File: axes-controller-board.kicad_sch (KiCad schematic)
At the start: 58 parts, among them IC1 TPS5450QDDARQ1, J10 Conn_01x08, J11 Conn_01x04, J12 Conn_01x08, J13 Conn_01x04, J14 Conn_01x08, J15 Conn_01x08, J16 Conn_01x04, J17 Conn_01x08, J18 Conn_01x08, J19 Conn_01x04, J2 Conn_01x03, J20 Conn_01x08, J21 Conn_01x08, J22 Conn_01x04, J23 Conn_01x08, J24 Conn_01x08, J25 Conn_01x04, J26 Conn_01x08, J27 Raspberry_Pi_2_3, J28 DC1, J29 DC2, J3 Conn_01x03, J30 DC3, J31 Conn_01x08, J32 Conn_01x08, J4 Conn_01x03, J5 DRIVER, J6 NTC, J7 DRIVER, J8 NTC, J9 Conn_01x08, U1 LM1117MP-3.3

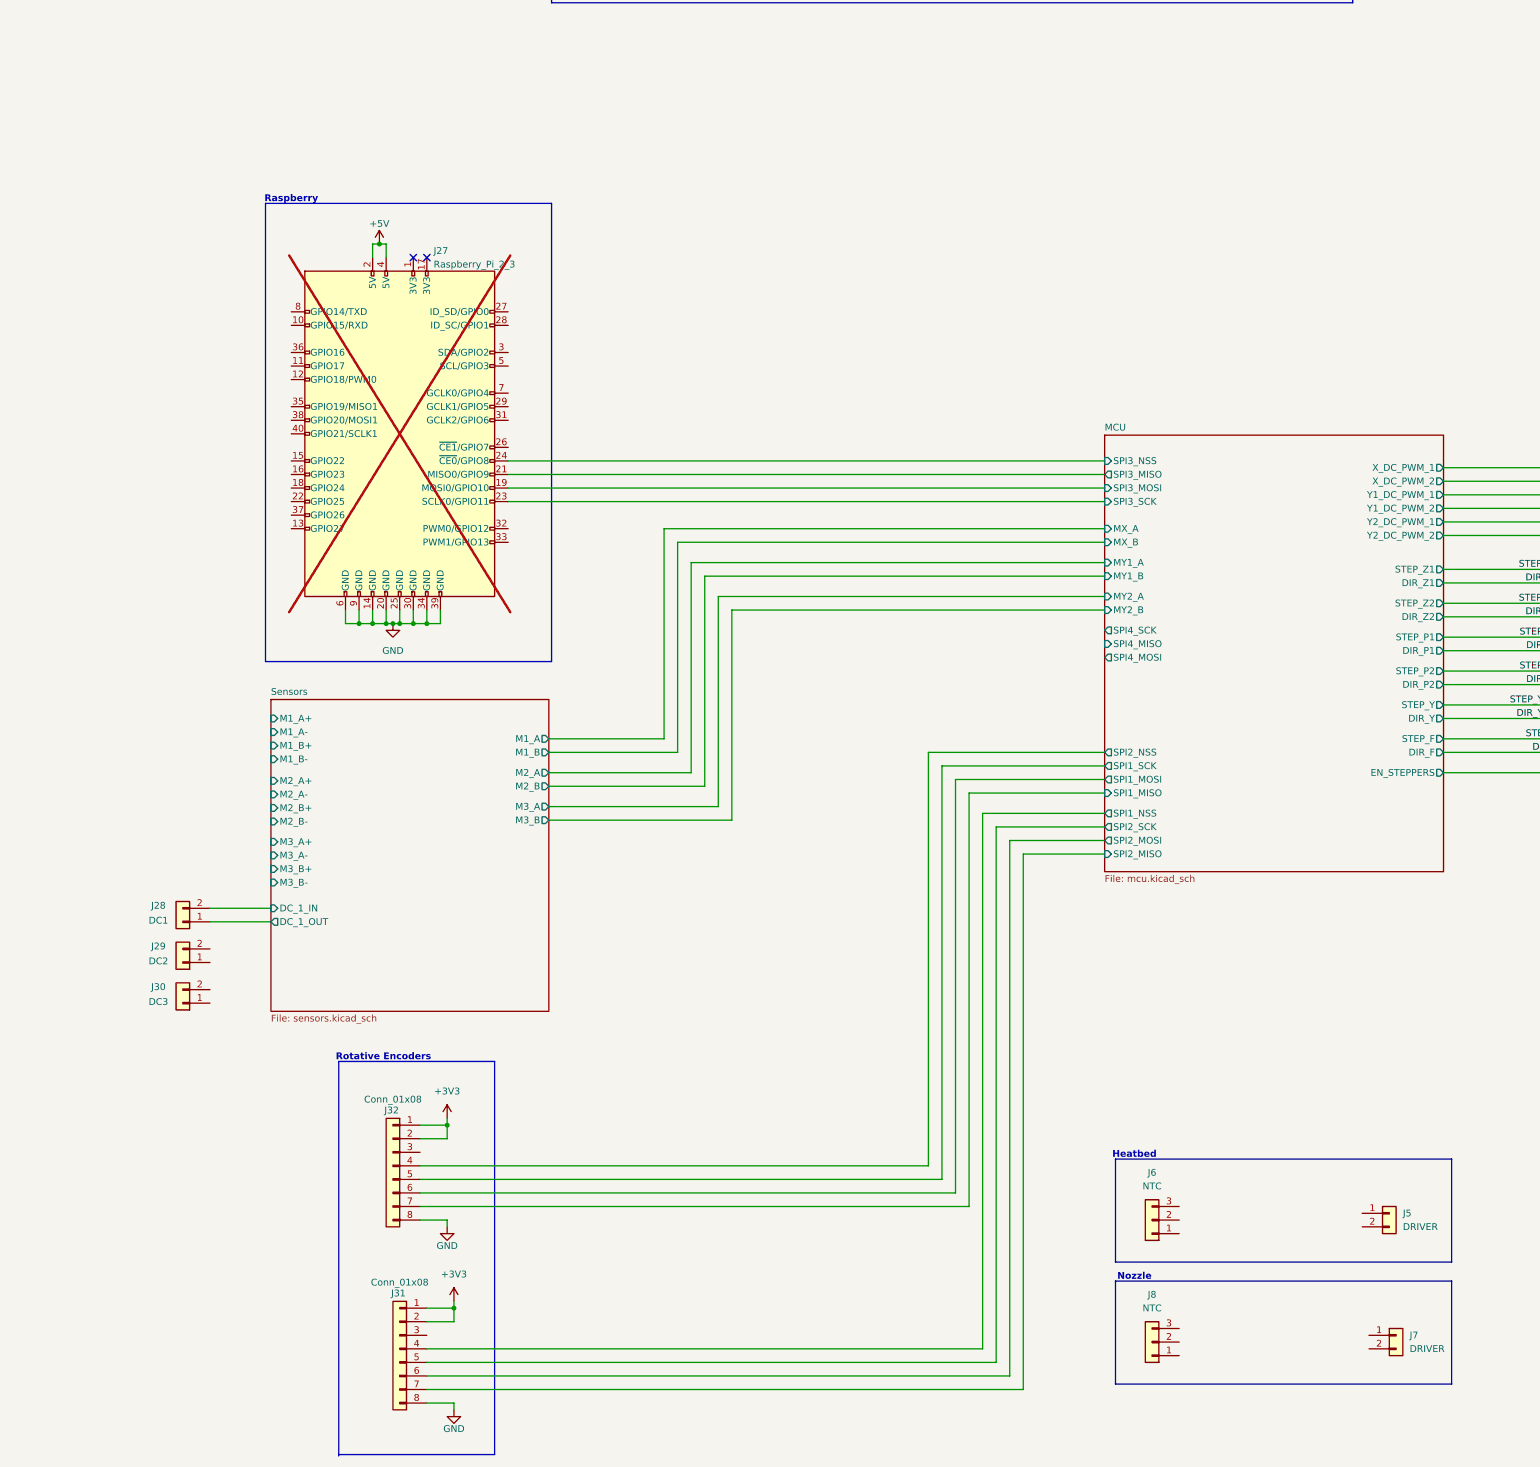
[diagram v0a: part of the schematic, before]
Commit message: feat: current sensor setup
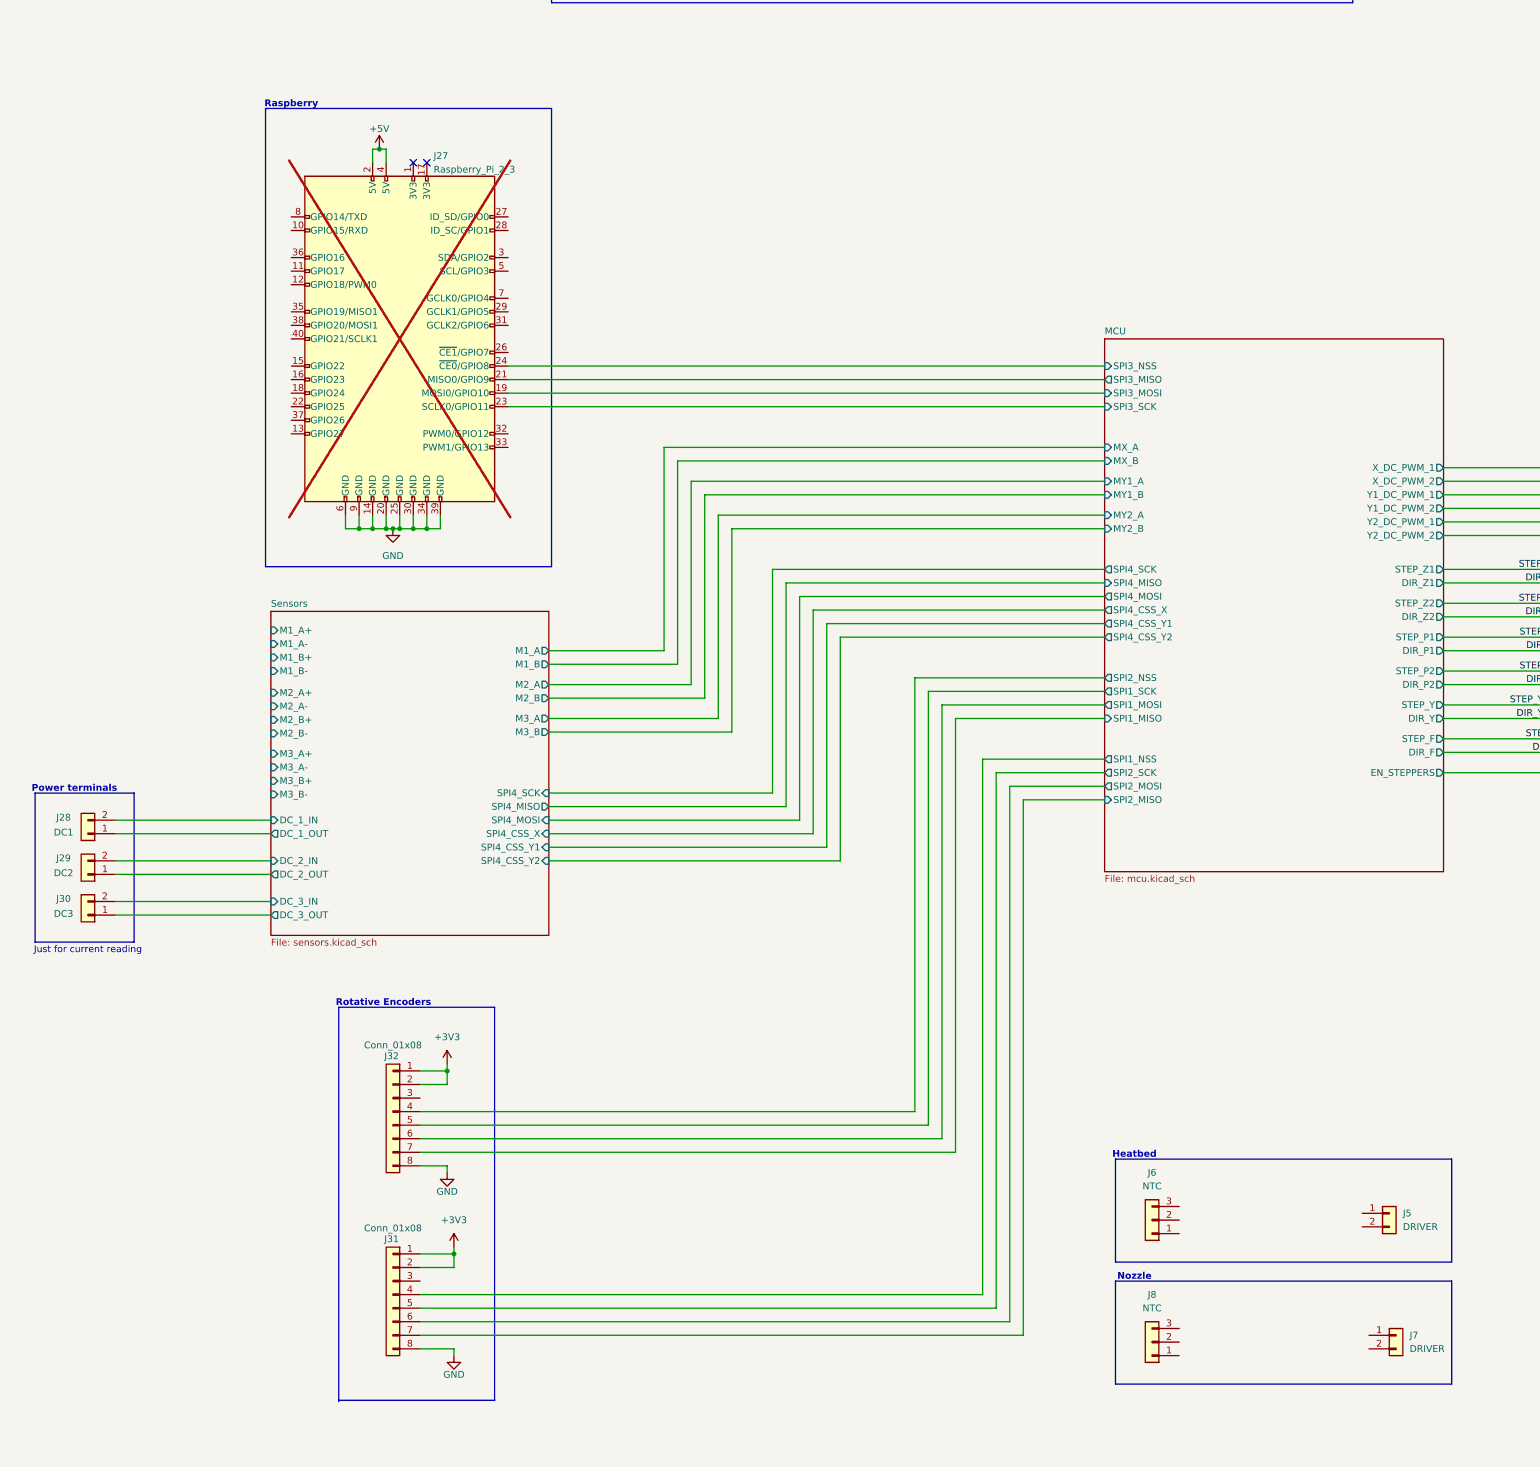
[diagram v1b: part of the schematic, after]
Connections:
- net Sensors/DC_3_OUT: now reaches J30.1 (Pin_1)
- net Sensors/DC_3_IN: now reaches J30.2 (Pin_2)
- net Sensors/DC_2_OUT: now reaches J29.1 (Pin_1)
- net Sensors/DC_2_IN: now reaches J29.2 (Pin_2)
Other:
- sheet MCU ports: added SPI4_CSS_X, SPI4_CSS_Y1, SPI4_CSS_Y2; removed none
- sheet Sensors ports: added DC_2_IN, DC_2_OUT, DC_3_IN, DC_3_OUT, SPI4_CSS_X, SPI4_CSS_Y1, SPI4_CSS_Y2, SPI4_MISO, SPI4_MOSI, SPI4_SCK; removed none
- note added: "Just for current reading"
- note added: "Power terminals"
- moved on the sheet: J27, J28, J29, J30, J31, J32
